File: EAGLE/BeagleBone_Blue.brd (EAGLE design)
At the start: 86.4 x 54.6 mm, 310 parts, among them J2 SERVO_HEADERS_8X, M1 JST_ZH_2, M2 JST_ZH_2, M3 JST_ZH_2, M4 JST_ZH_2, Q1 MOSFET-N, U1 TCAN1051HV, U10 TXS0108ERGYR, U13 EMMC, U2 SN74LV1T126DBVR, U3 TPD4S012DRY, U4 TPD4S012DRY, U5 24LC_32AT-I/OT, U6 SN74LVC1G07_DCK_5, U7 WL1835MODGBMOCT, U8 TPS2105_DBV_5, U9 TXS0108ERGYR, X2 SCHA5B0200, X3 USB1, X4 10118192-0001LF, Y1 24 MHz, Y2 32.768kHz

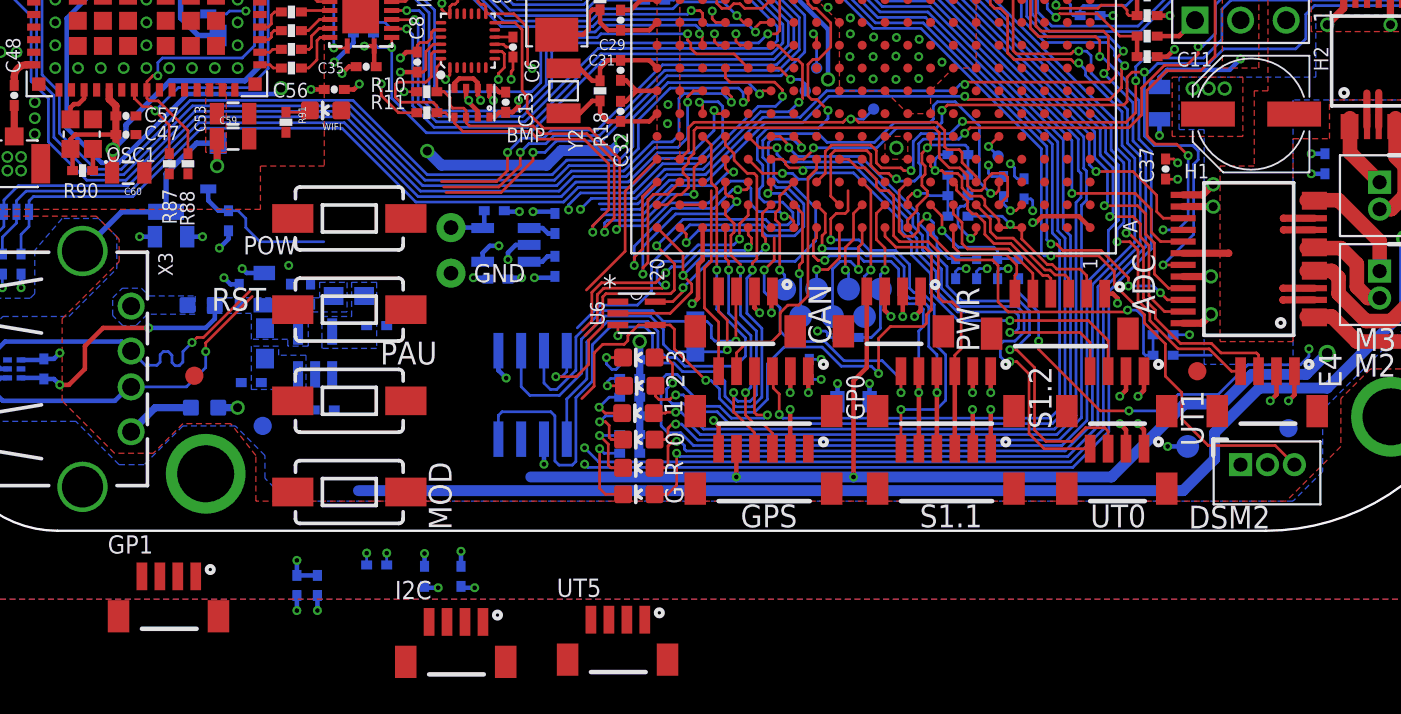
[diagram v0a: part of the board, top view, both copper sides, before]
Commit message: Updated placement
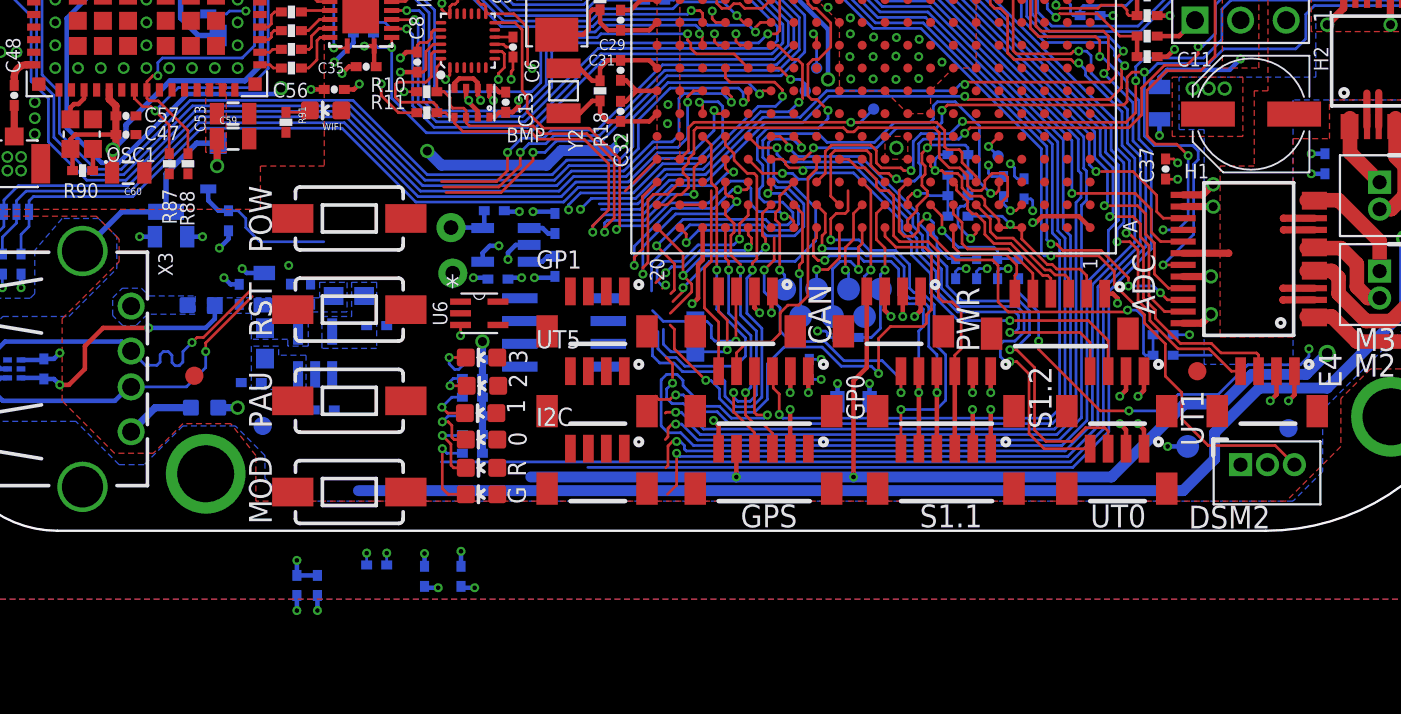
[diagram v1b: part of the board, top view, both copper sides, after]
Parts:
- moved GP1 28.7 mm to (37.5, -42.5)
- moved UT5 13.9 mm to (37.5, -47.0)
- moved I2C 12.5 mm to (37.5, -51.3)
- moved 2 8.76 mm to (30.0, -46.5)
- moved 0 8.76 mm to (30.0, -49.5)
- moved 1 8.76 mm to (29.9, -48.1)
- moved 3 8.76 mm to (30.0, -45.0)
- moved G 8.76 mm to (30.0, -52.6)
- moved R 8.76 mm to (30.0, -51.1)
- moved R21 8.76 mm to (29.5, -49.3)
- moved R22 8.76 mm to (29.5, -50.3)
- moved R61 8.76 mm to (29.5, -48.2)
- moved R62 8.76 mm to (29.5, -47.2)
- moved R63 8.76 mm to (29.5, -46.1)
- moved R64 8.76 mm to (29.5, -45.1)
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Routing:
- net DCAN1_RX: track 44.6 -> 25.2 mm
- net CANL: track 21.4 -> 8.07 mm
- net DCAN1_SILENT: track 46.5 -> 34.5 mm, vias 3 -> 2
- net CANH: track 19.6 -> 8.70 mm
- net DCAN1_TX: track 30.2 -> 19.7 mm
- net RESET: track 40.1 -> 32.3 mm
- net PAUSE_BTN: track 69.3 -> 76.9 mm, vias 2 -> 1
- net POWER_BTN: track 8.92 -> 2.51 mm
- net I2C1_SDA: track 16.1 -> 9.75 mm
- net I2C1_SCL: track 14.0 -> 7.93 mm
- net N$75: track 27.9 -> 22.9 mm
- net PMIC_PGOOD: track 16.9 -> 14.0 mm
- net 3.3V: track 138.6 -> 136.9 mm, vias 61 -> 60
- net GND: track 232.2 -> 230.8 mm, vias 212 -> 211
- net VDD_RTC: track 20.3 -> 19.3 mm
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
